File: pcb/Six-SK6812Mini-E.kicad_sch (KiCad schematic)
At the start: 12 parts

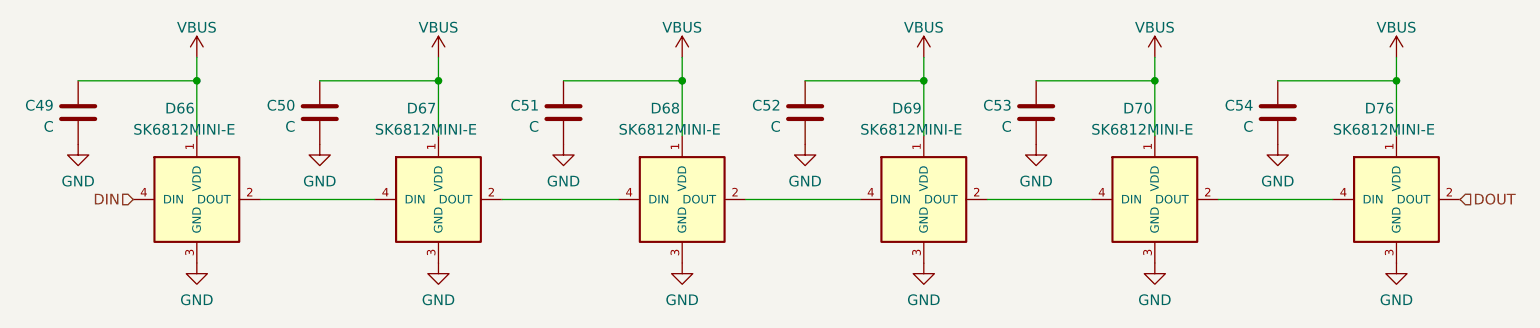
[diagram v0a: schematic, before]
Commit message: Update kicad schematics
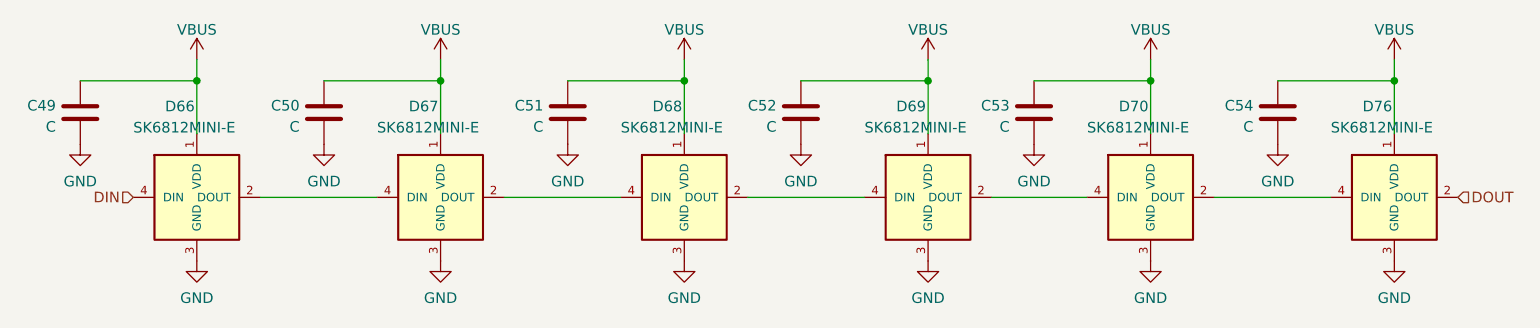
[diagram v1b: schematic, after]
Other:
- moved on the sheet: C50, C51, C52, D69, D70
